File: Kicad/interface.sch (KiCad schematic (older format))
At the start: 16 parts, among them SW1 Push, SW10 Push, SW11 Push, SW12 Push, SW2 Push, SW3 Push, SW4 Push, SW5 Push, SW6 Push, SW7 Push, SW8 Push, SW9 Push, U1 TLC59281DBQ

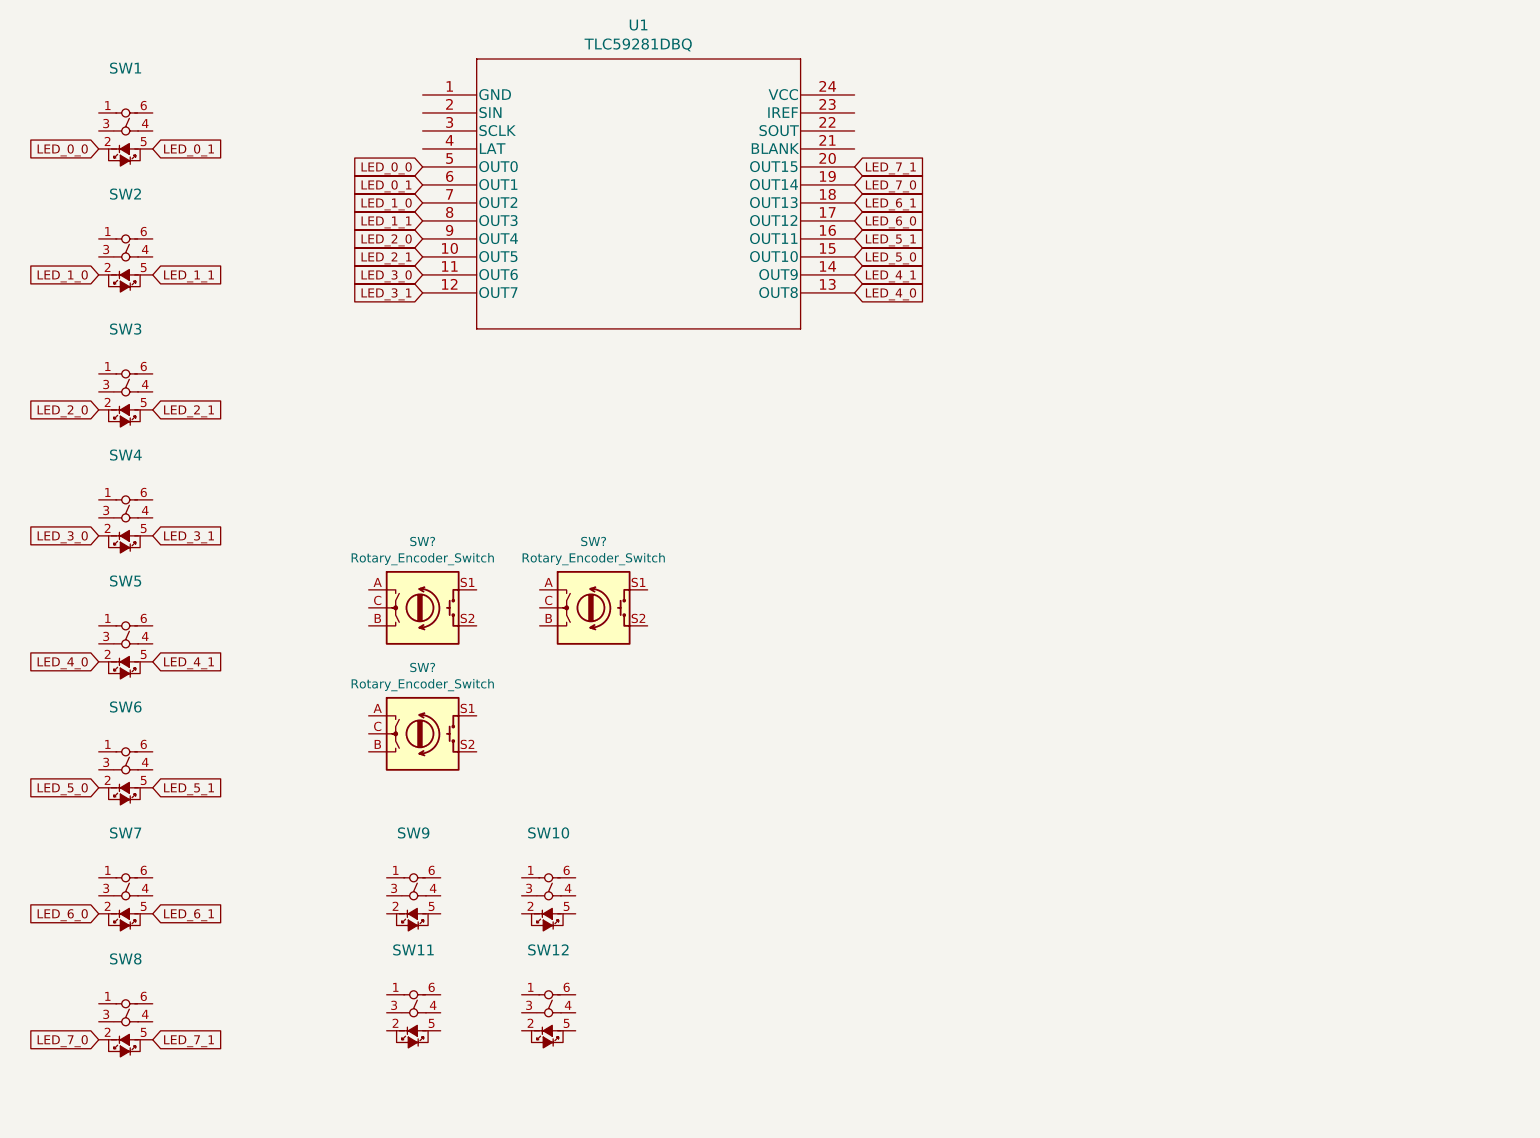
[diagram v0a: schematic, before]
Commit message: making progress on interface
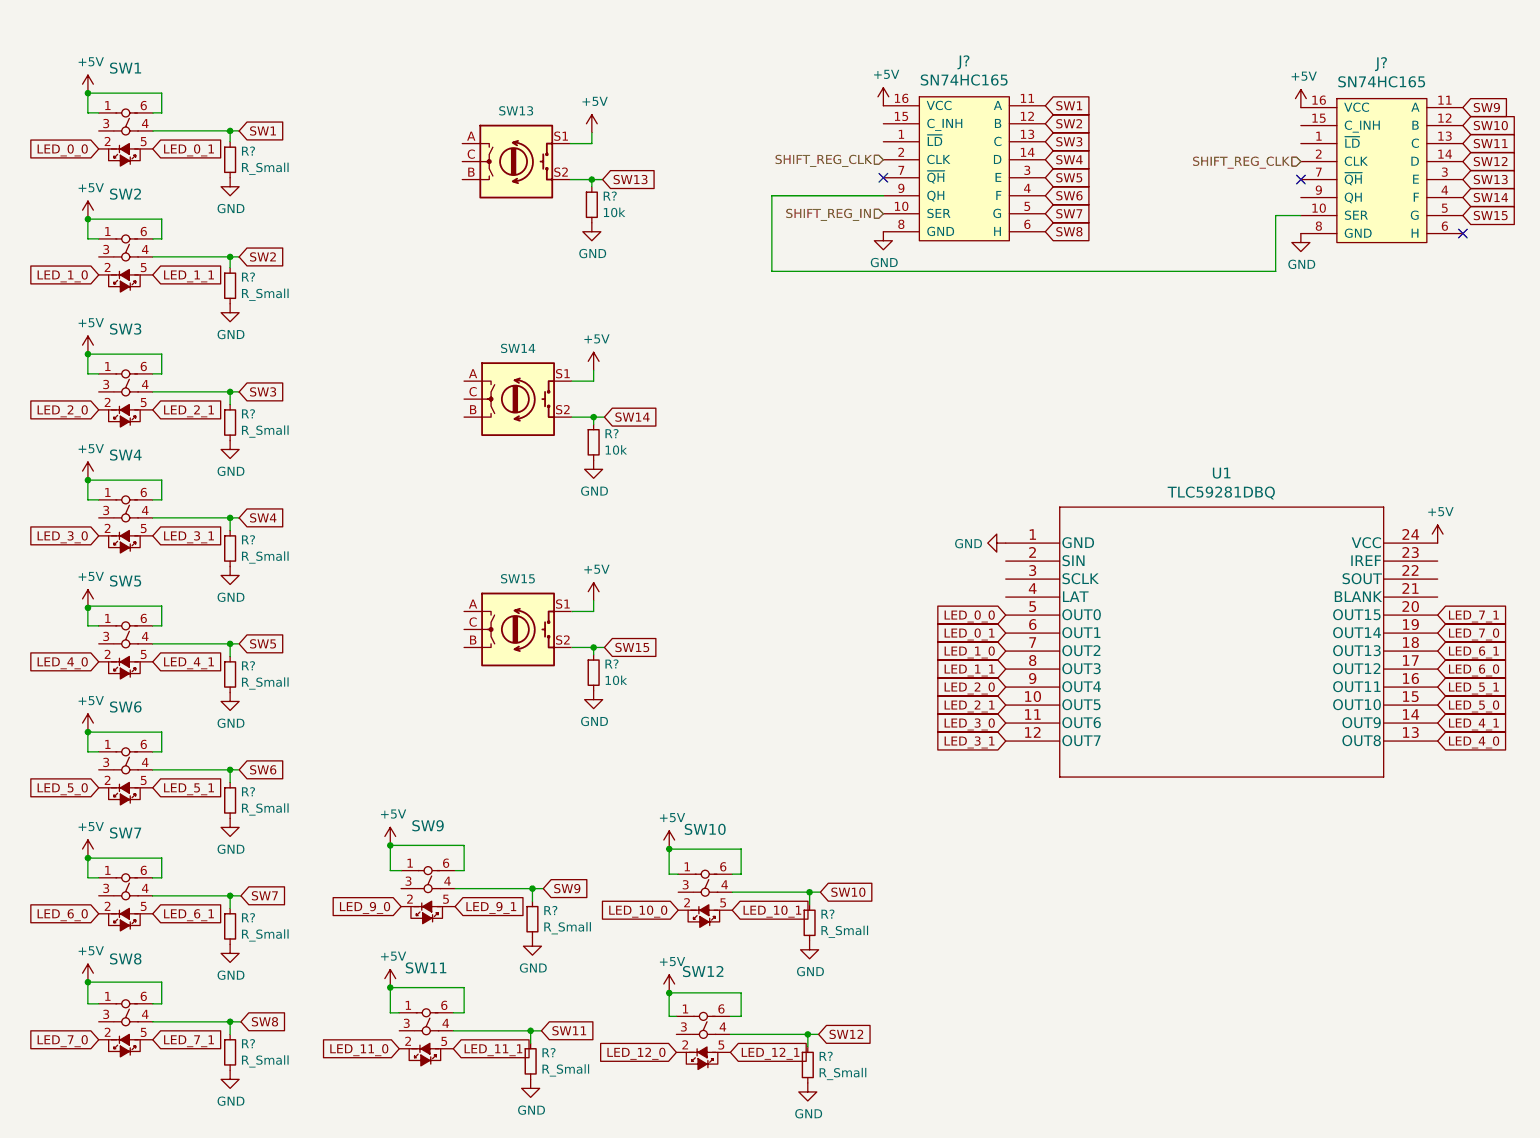
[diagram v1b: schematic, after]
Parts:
- removed SW? (x2): Rotary_Encoder_Switch, Rotary_Encoder:RotaryEncoder_Alps_EC12E-Switch_Vertical_H20mm, symbol Device:Rotary_Encoder_Switch
- added J? (x2): SN74HC165, symbol eurocad:SN74HC165
- added R? (x12): R_Small, symbol Device:R_Small
- added R? (x3): 10k, symbol Device:R_Small
- added SW13, SW14: Rotary_Encoder_Switch, Rotary_Encoder:RotaryEncoder_Alps_EC12E-Switch_Vertical_H20mm, symbol Device:Rotary_Encoder_Switch
- gave numbers to parts that had none: 1
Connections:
- net +5V: now reaches SW15.S1
- net +5V: now also SW1.1, SW1.6, SW10.1, SW10.6, SW11.1, SW11.6, SW12.1, SW12.6, SW2.1, SW2.6, SW3.1, SW3.6, SW4.1, SW4.6, SW5.1, SW5.6, SW6.1, SW6.6, SW7.1, SW7.6, SW8.1, SW8.6, SW9.1, SW9.6, U1.24 (VCC), J?.16 (VCC), J?.16 (VCC), SW13.S1, SW14.S1
- net SW15: now reaches SW15.S2
- net SW15: now also J?.5 (G), R?.1
- net SW5: now reaches SW5.4
- net SW5: now also J?.3 (E), R?.1
- net SW6: now reaches SW6.4
- net SW6: now also J?.4 (F), R?.1
- net SW3: now reaches SW3.4
- net SW3: now also J?.13 (C), R?.1
- net SW4: now reaches SW4.4
- net SW4: now also J?.14 (D), R?.1
- net LED_11_0: now reaches SW11.2
- net SW11: now reaches SW11.4
- net SW11: now also J?.13 (C), R?.1
- net LED_11_1: now reaches SW11.5
- net LED_12_0: now reaches SW12.2
- net SW12: now reaches SW12.4
- net SW12: now also J?.14 (D), R?.1
- net LED_12_1: now reaches SW12.5
- net GND: now reaches U1.1 (GND)
- net GND: now also J?.8 (GND), J?.8 (GND), R?.2, R?.2, R?.2, R?.2, R?.2, R?.2, R?.2, R?.2, R?.2, R?.2, R?.2, R?.2, R?.2, R?.2, R?.2
- net LED_10_0: now reaches SW10.2
- net SW10: now reaches SW10.4
- net SW10: now also J?.12 (B), R?.1
- net LED_10_1: now reaches SW10.5
- net SW2: now reaches SW2.4
- net SW2: now also J?.12 (B), R?.1
- net LED_9_0: now reaches SW9.2
- net SW9: now reaches SW9.4
- net SW9: now also J?.11 (A), R?.1
- net LED_9_1: now reaches SW9.5
- net SW8: now reaches SW8.4
- net SW8: now also J?.6 (H), R?.1
- net SW7: now reaches SW7.4
- net SW7: now also J?.5 (G), R?.1
- net SW1: now reaches SW1.4
- net SW1: now also J?.11 (A), R?.1
- new net: J?.10 (SER), J?.9 (QH)
- new net SHIFT_REG_CLK: J?.2 (CLK), J?.2 (CLK)
- new net SHIFT_REG_IN: J?.10 (SER)
- new net SW13: J?.3 (E), R?.1, SW13.S2
- new net SW14: J?.4 (F), R?.1, SW14.S2
- no-connect marks 0 -> 3
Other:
- moved on the sheet: SW10, SW11, SW12, SW15, SW9, U1
